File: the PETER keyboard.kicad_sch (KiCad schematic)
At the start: 16 parts

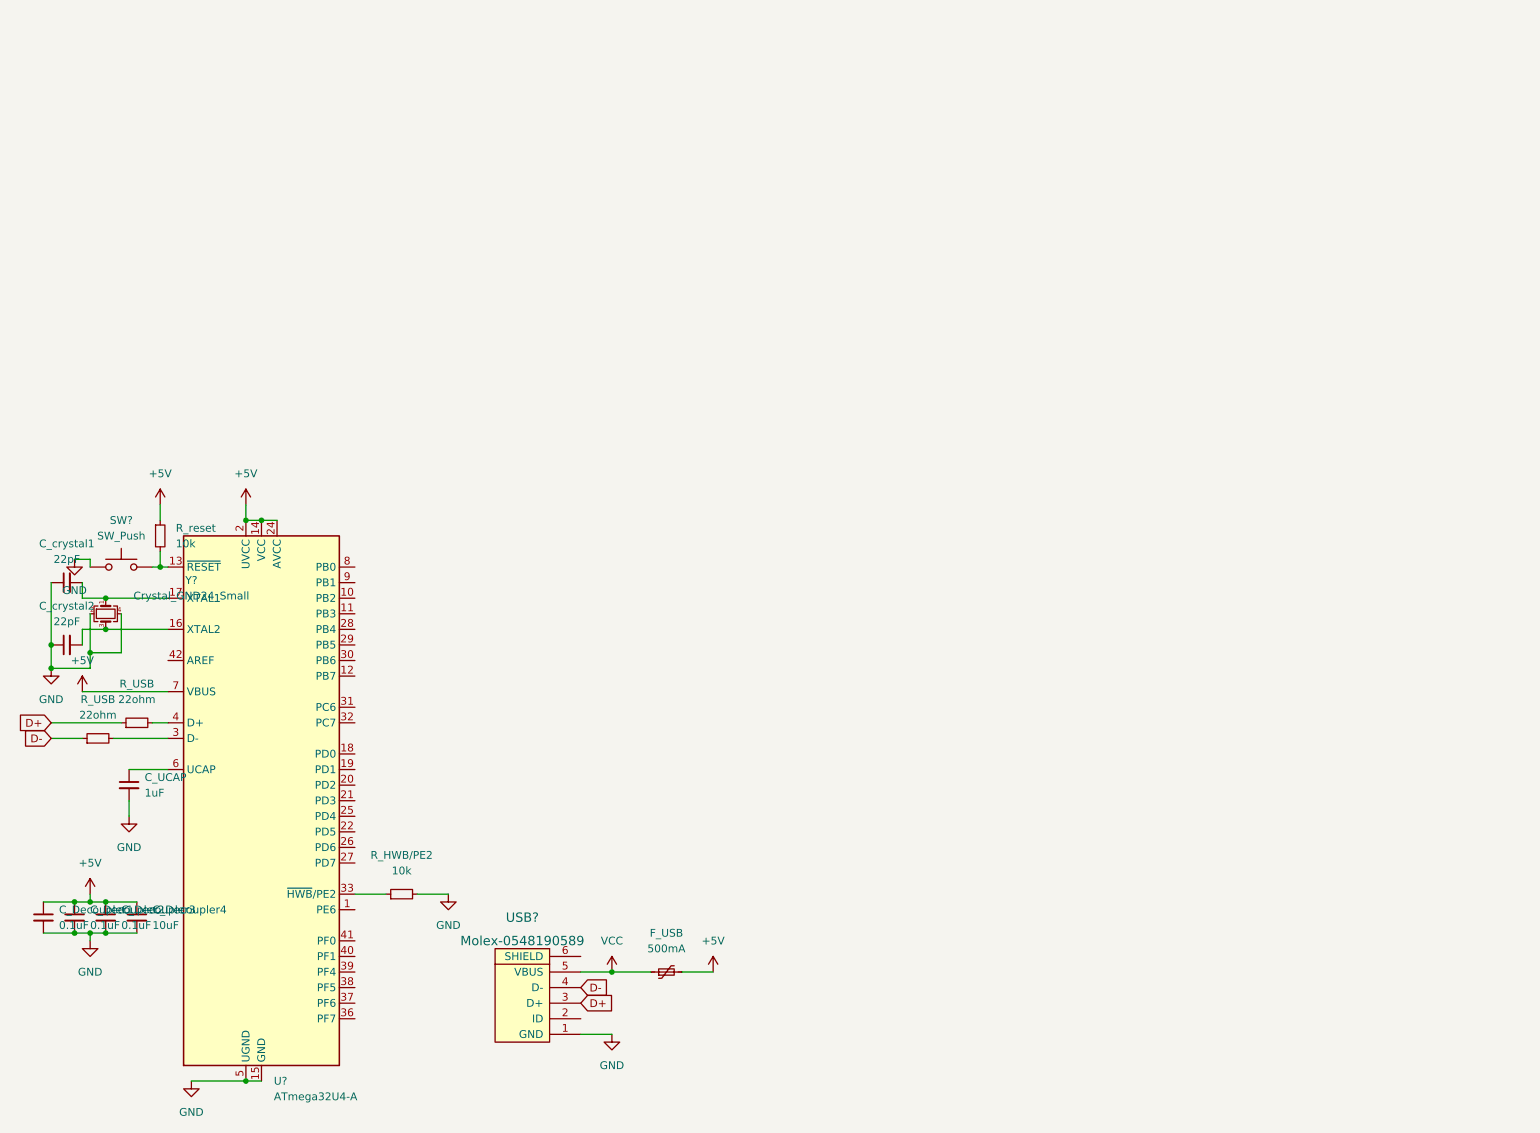
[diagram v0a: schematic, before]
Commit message: starting to set up matrix
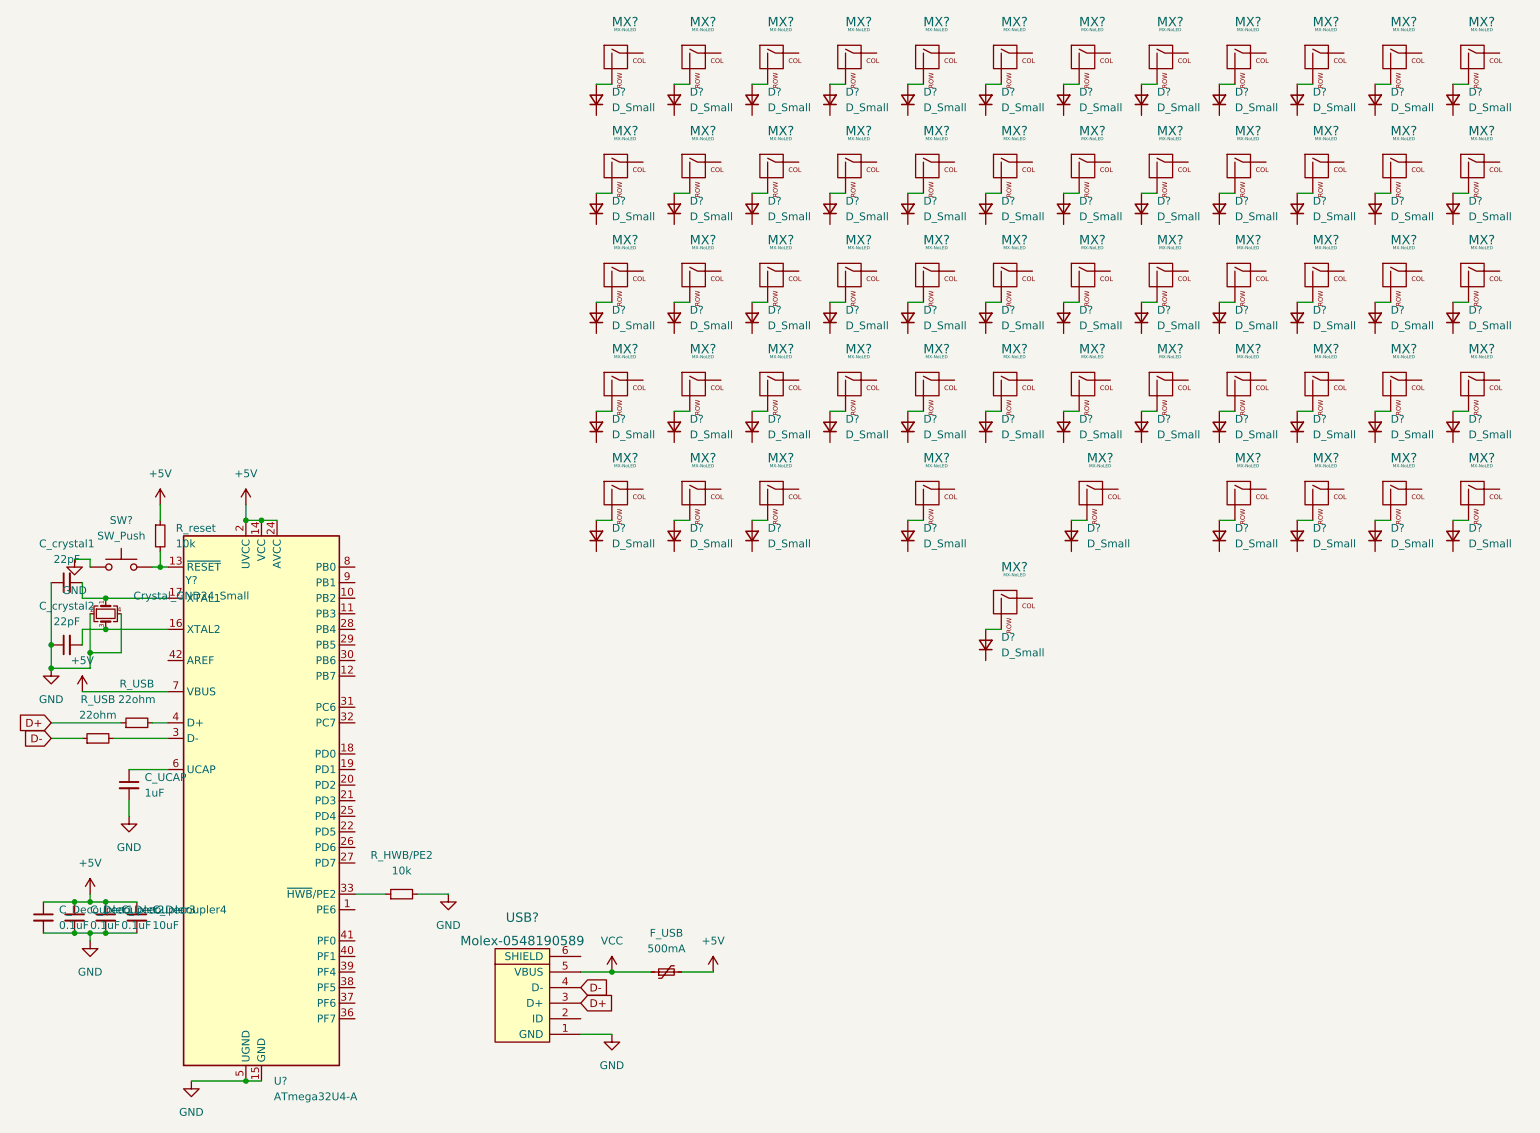
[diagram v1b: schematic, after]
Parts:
- added D? (x58): D_Small, symbol Device:D_Small
- added MX? (x58): MX-NoLED, symbol MX_Alps_Hybrid:MX-NoLED
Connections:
- new net: D?.2 (A), MX?.2 (ROW) (x58)
